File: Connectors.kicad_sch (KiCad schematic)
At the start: 21 parts, among them J1 353630460, J3 2171750001, J4 353630660, J5 353630660, U4 TJA1051T/3, U5 ICM-42688-P

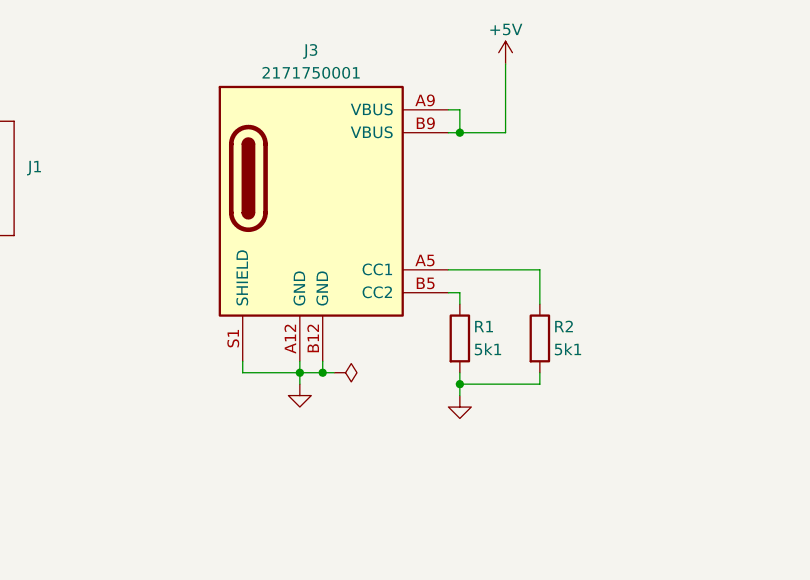
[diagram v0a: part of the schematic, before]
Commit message: update pcb
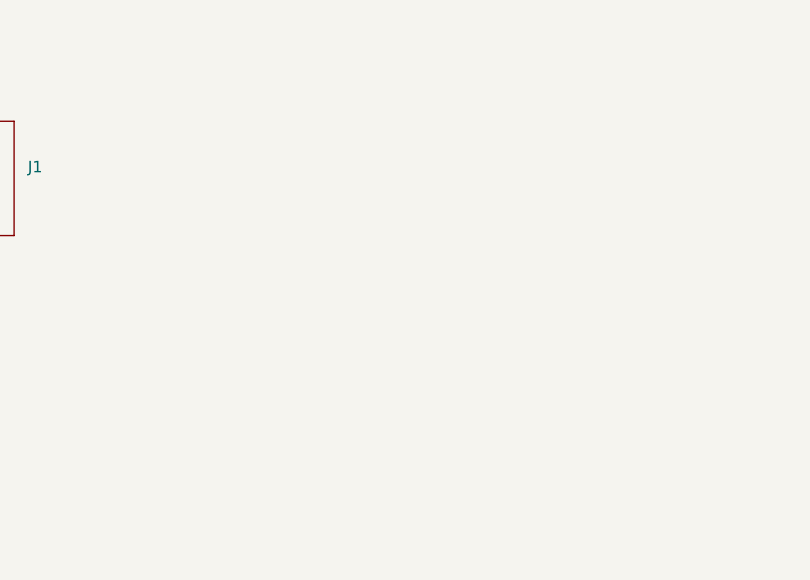
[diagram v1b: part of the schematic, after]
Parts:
- removed J3: 2171750001, common:molex_2171750001_usb_c_6p, symbol common:molex_2171750001_usb_c_6p
- removed R1, R2: 5k1, Resistor_SMD:R_0603_1608Metric, symbol Device:R
